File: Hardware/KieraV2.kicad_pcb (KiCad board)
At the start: 2 copper layers, 121.7 x 50.3 mm, 87 parts, among them J1 Conn_01x04_Male, J2 Conn_01x05_Male, SW1 SW_Rotary2x4, SW2 SW_Rotary2x4, SW3 SW_Push, SW4 SW_Push, SW5 SW_Push, SW6 SW_Push, SW7 SW_MEC_5G, U1 STM32L4P5RET6, U2 LM1117-3.3, U3 IMS330DHCX, U4 ATA6561-GAQW-N, Y1 Crystal_GND24

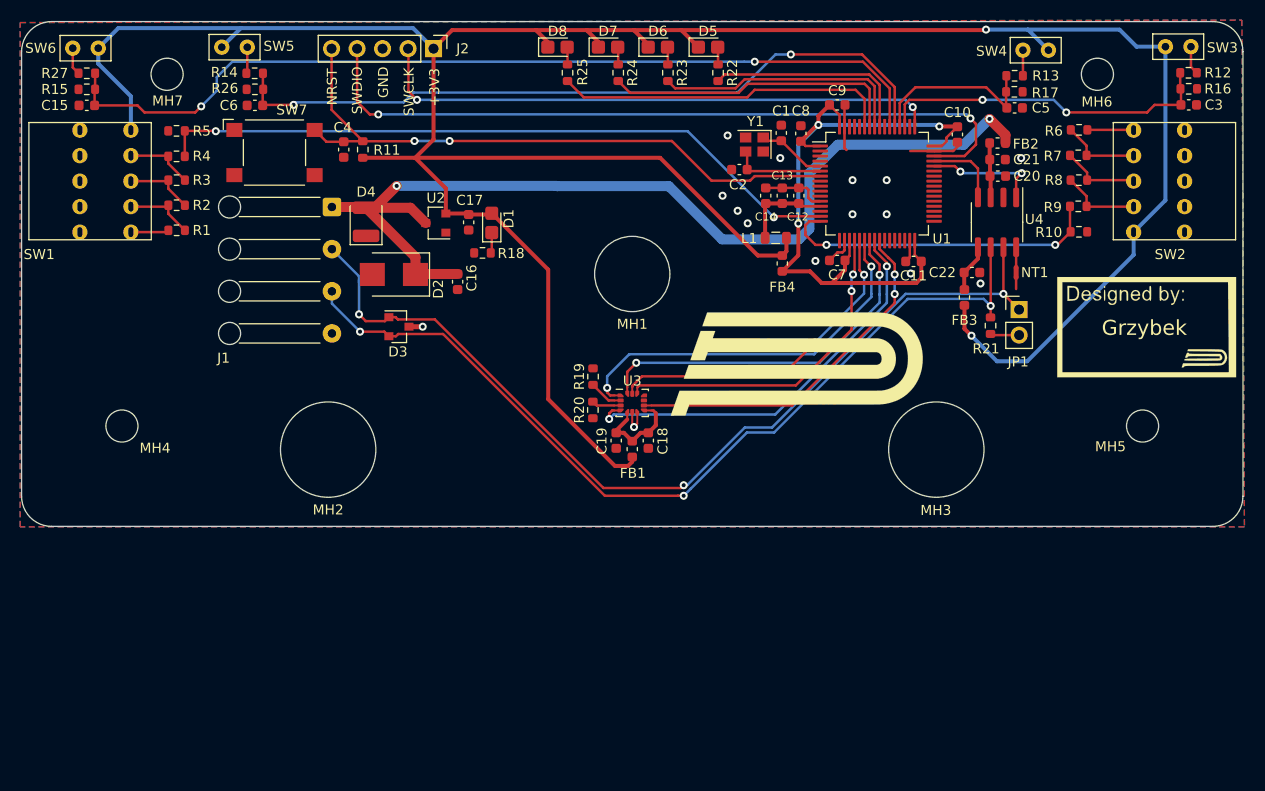
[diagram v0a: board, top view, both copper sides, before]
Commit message: pcb changed
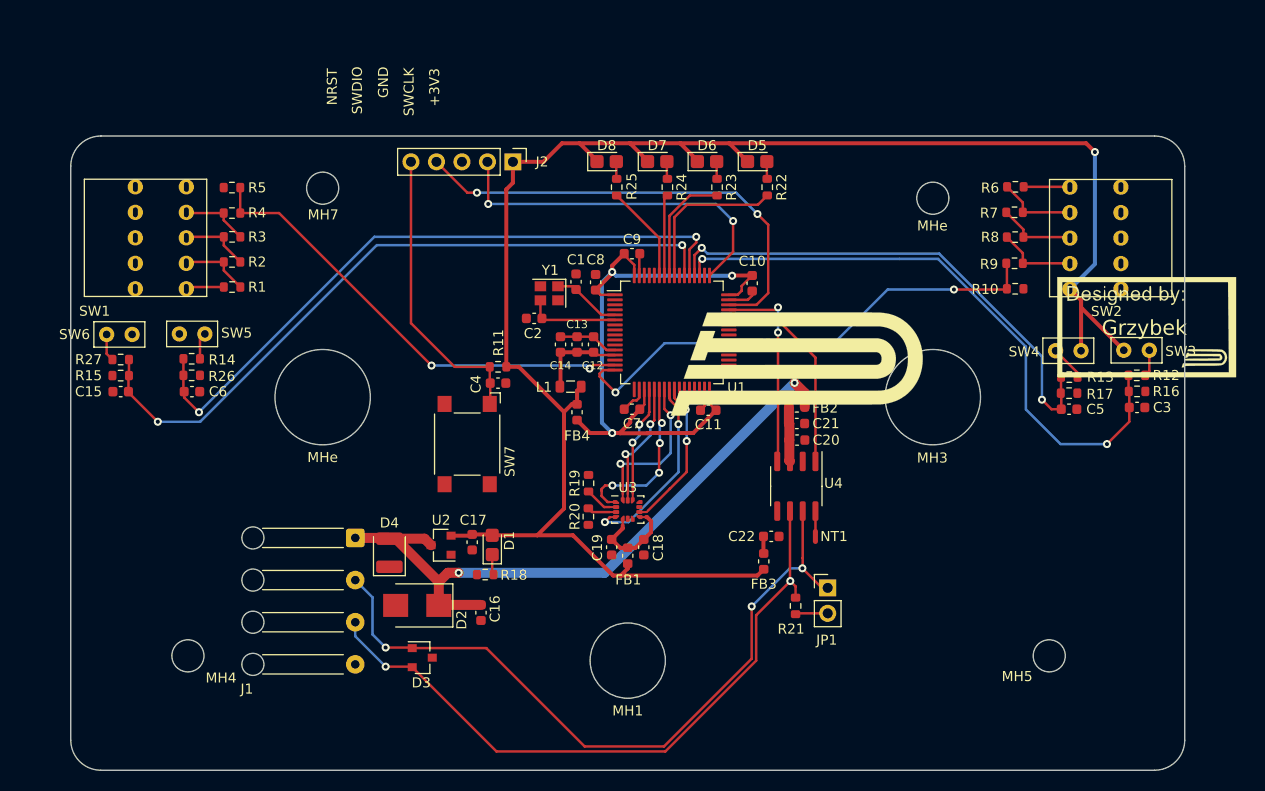
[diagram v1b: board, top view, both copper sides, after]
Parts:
- removed MH6: MountingHole_3.2mm_M3, MountingHole:MountingHole_3.2mm_M3
- added MHe: MountingHole_3.2mm_M3, MountingHole:MountingHole_3.2mm_M3, F.Cu at (188.4, 96.0)
- moved MH1 38.5 mm to (158.0, 142.1)
- moved SW7 34.8 mm to (142.0, 120.5), turned to 270 degrees
- moved R21 34.0 mm to (174.7, 136.6)
- moved JP1 33.7 mm to (177.9, 134.8)
- moved C16 33.1 mm to (143.4, 137.3)
- moved D2 33.1 mm to (137.0, 136.6)
- moved D3 33.1 mm to (137.5, 141.8)
- moved D4 33.1 mm to (134.2, 131.3)
- moved J1 33.1 mm to (130.8, 129.8)
- moved C20 33.0 mm to (174.9, 120.1)
- moved C21 33.0 mm to (174.8, 118.5)
- moved FB2 33.0 mm to (174.8, 116.8)
- moved FB3 33.0 mm to (171.6, 132.2)
- moved U4 33.0 mm to (174.8, 124.7)
- moved C22 33.0 mm to (172.3, 129.7)
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- renumbered MH2 to MHe
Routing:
- net +3V3: track 284.5 -> 177.4 mm, vias 2 -> 1
- net /NRST: track 63.2 -> 29.5 mm, vias 2 -> 0
- net /SW4: track 17.8 -> 51.3 mm, vias 0 -> 2
- net +5V: track 99.4 -> 67.6 mm
- net /SWDIO: track 74.6 -> 46.9 mm
- net /SW3: track 34.0 -> 61.2 mm
- net /ControlLED4: track 33.7 -> 9.74 mm
- net /SW1: track 69.5 -> 46.4 mm
- net /CAN-: track 90.4 -> 68.0 mm, vias 3 -> 2
- net /CAN+: track 95.3 -> 73.0 mm
- net /ControlLED3: track 29.9 -> 8.10 mm
- net /IMU_INT1: track 41.0 -> 19.3 mm
- net /IMU_SPI1_CS: track 33.4 -> 11.8 mm
- net /SWCLK: track 57.2 -> 35.7 mm
- net /IMU_SPI1_MISO: track 38.6 -> 17.3 mm, vias 2 -> 4
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- removed copper zone on B.Cu, net GND
- removed copper zone on F.Cu, net GND
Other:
- board size 121.7 x 50.3 mm -> 111 x 63.2 mm
